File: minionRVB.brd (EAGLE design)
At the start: 100.3 x 100 mm, 128 parts, among them IC1 74HCT245DW

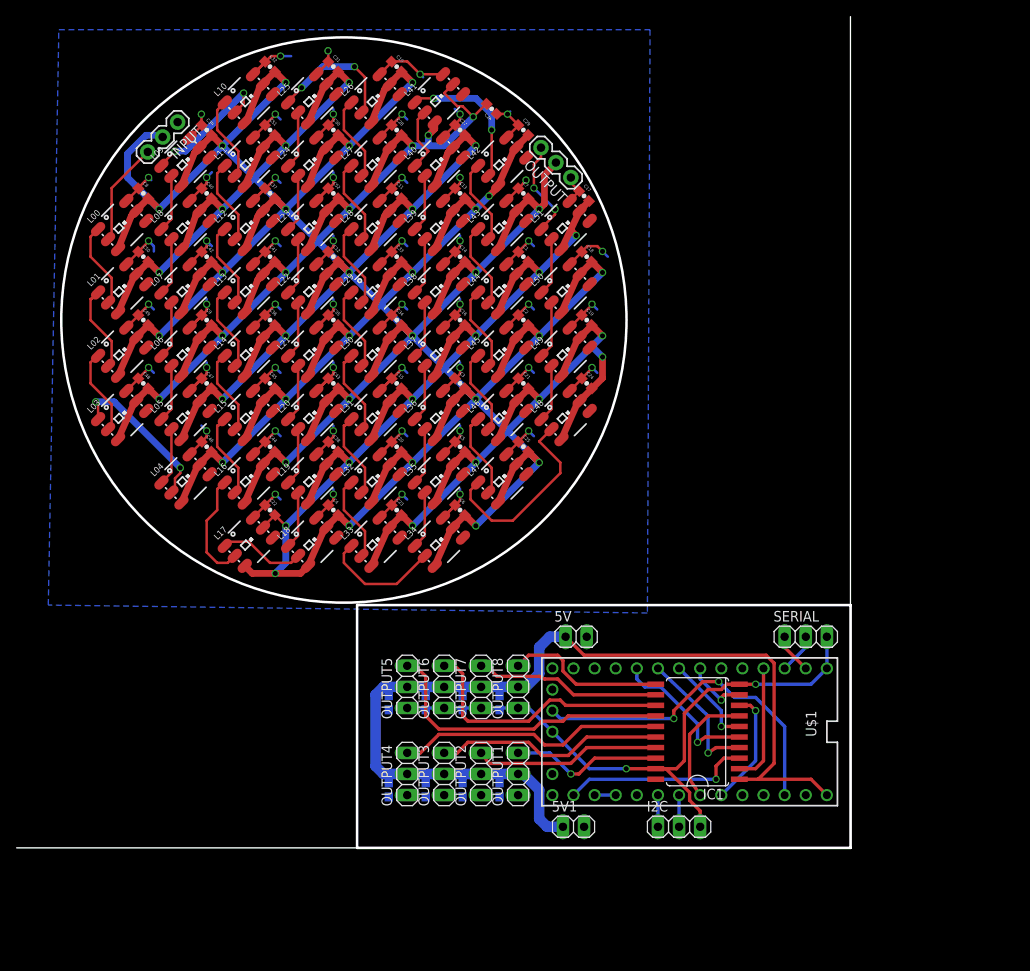
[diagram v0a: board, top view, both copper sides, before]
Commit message: move boards
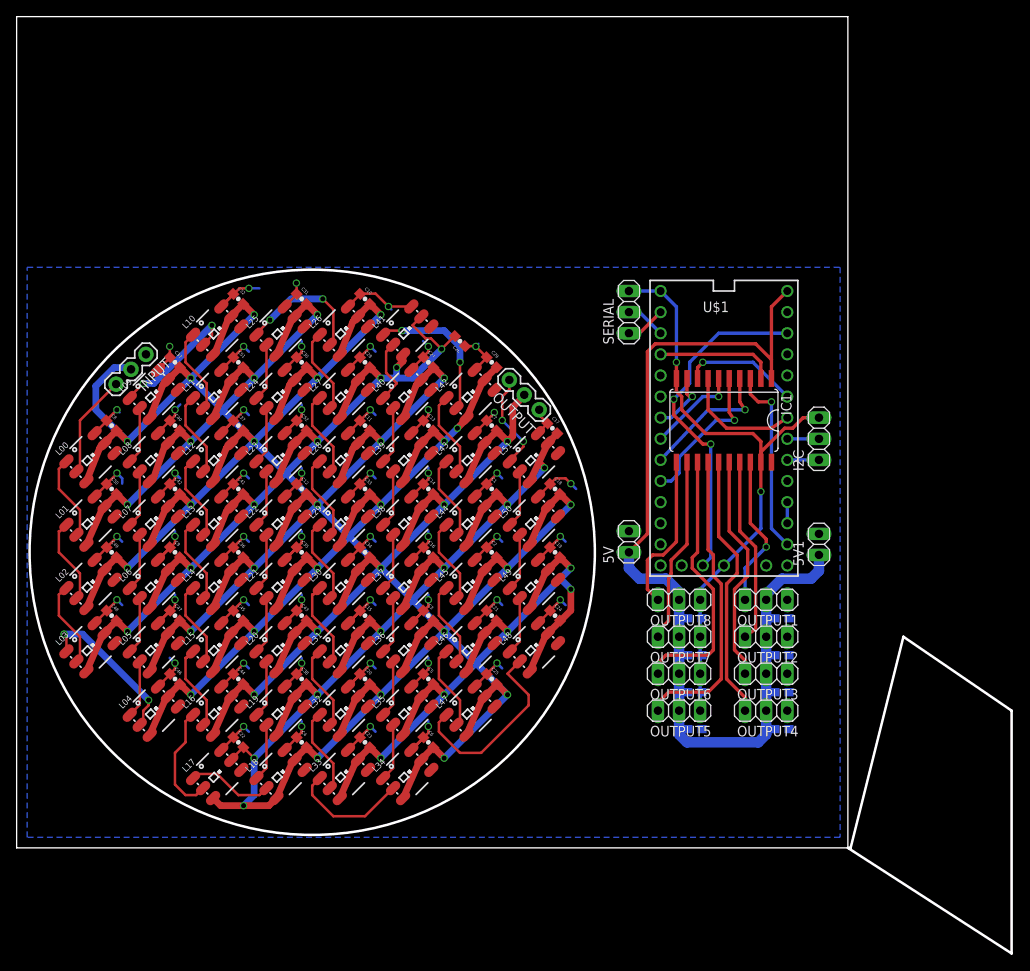
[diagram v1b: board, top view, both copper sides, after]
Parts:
- moved I2C 49.6 mm to (96.5, 49.2), turned to 90 degrees
- moved C56 47.9 mm to (92.1, 14.3), turned to 0 degrees
- moved 5V1 45.0 mm to (96.5, 36.5), turned to 90 degrees
- moved SERIAL 44.5 mm to (73.7, 64.5), turned to 90 degrees
- moved C53 44.4 mm to (92.1, 18.7), turned to 0 degrees
- moved OUTPUT4 43.8 mm to (90.2, 16.5), turned to 180 degrees
- moved C54 41.7 mm to (92.1, 23.2), turned to 0 degrees
- moved OUTPUT3 40.6 mm to (90.2, 21.0), turned to 180 degrees
- moved C55 39.7 mm to (92.1, 27.6), turned to 0 degrees
- moved OUTPUT2 38.1 mm to (90.2, 25.4), turned to 180 degrees
- moved IC1 37.6 mm to (85.1, 51.4), turned to 180 degrees
- moved C58 37.0 mm to (81.6, 14.3), turned to 0 degrees
- moved U$1 36.7 mm to (85.1, 50.5), turned to 0 degrees
- moved OUTPUT1 36.5 mm to (90.2, 29.8), turned to 180 degrees
- moved OUTPUT5 32.8 mm to (79.7, 16.5), turned to 180 degrees
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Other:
- board size 100.3 x 100 mm -> 119.7 x 112.7 mm
